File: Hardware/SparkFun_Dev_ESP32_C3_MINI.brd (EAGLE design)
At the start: 17.8 x 33 mm, 44 parts, among them J1 USB Female Type C Connector, J5 Vertical Qwiic Connector, U2 RT9080-33GJ5

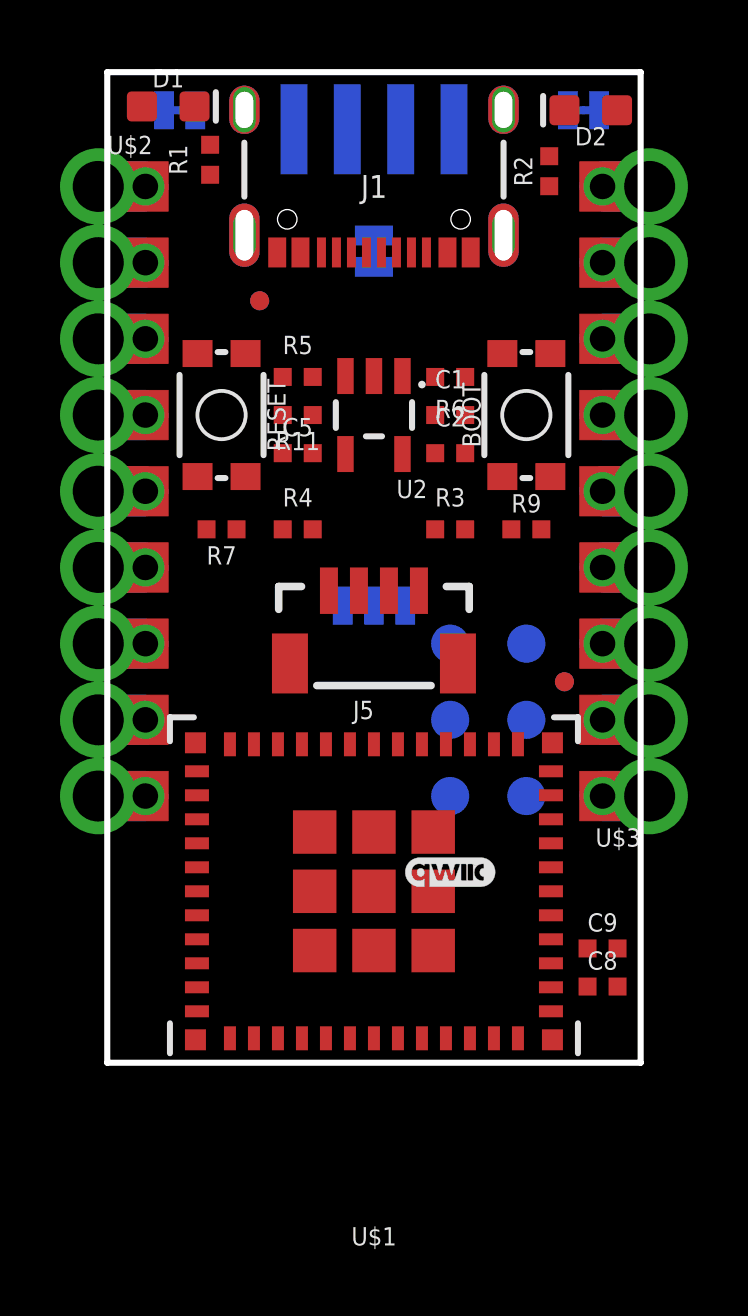
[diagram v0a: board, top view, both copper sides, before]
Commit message: Some updates to layout
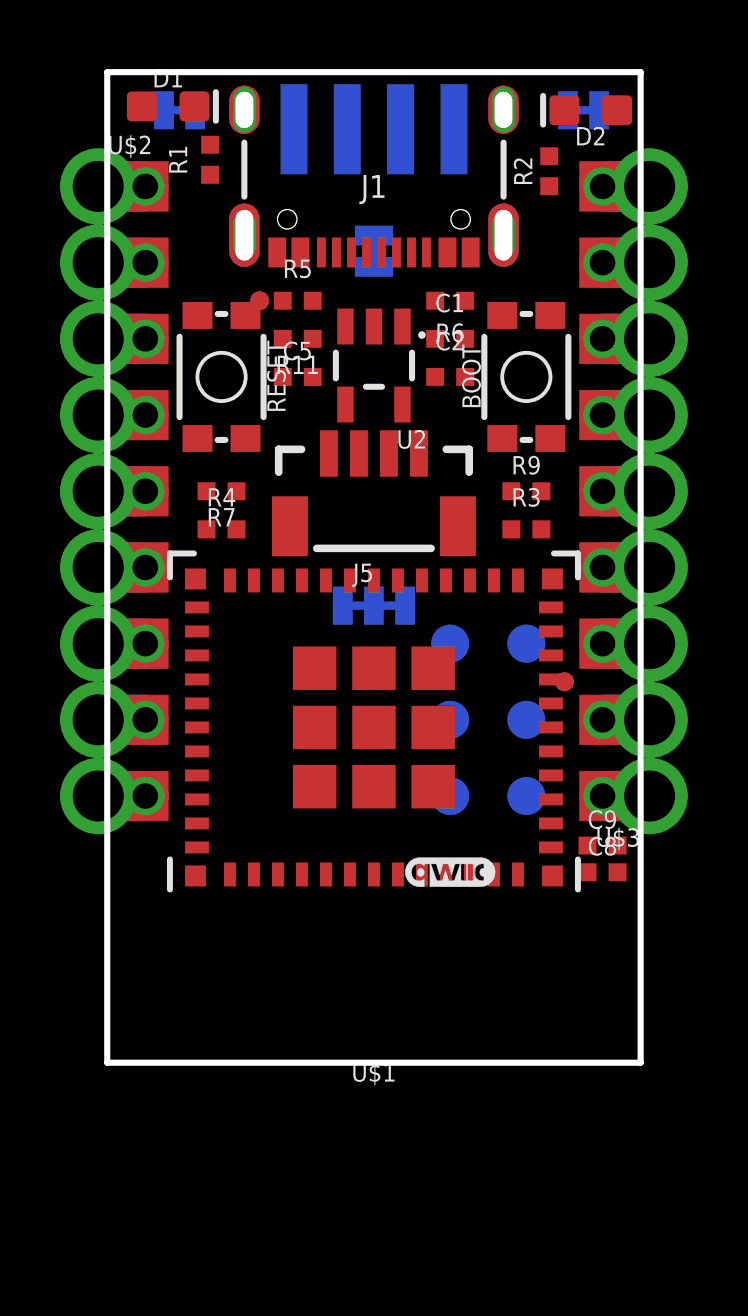
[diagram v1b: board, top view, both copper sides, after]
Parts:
- moved U$1 5.46 mm to (10.2, 11.2)
- moved J5 4.57 mm to (10.2, 21.1)
- moved C8 3.81 mm to (17.8, 6.35)
- moved C9 3.43 mm to (17.8, 7.24)
- moved R3 2.54 mm to (15.2, 17.8)
- moved R4 2.54 mm to (5.08, 17.8)
- moved C1 2.54 mm to (12.7, 24.1)
- moved C2 2.54 mm to (12.7, 22.9)
- moved C5 2.54 mm to (7.62, 22.9)
- moved R11 2.54 mm to (7.62, 24.1)
- moved R5 2.54 mm to (7.62, 25.4)
- moved R6 2.54 mm to (12.7, 25.4)
- moved U2 1.65 mm to (10.2, 23.2)
- moved BOOT 1.27 mm to (15.2, 22.9)
- moved R7 1.27 mm to (5.08, 19.1)
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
